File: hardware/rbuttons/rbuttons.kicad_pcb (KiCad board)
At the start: 2 copper layers, 62 x 105 mm, 8 parts, among them U1 SKRBAKE010, U2 SKRBAKE010, U3 SKRBAKE010, U4 SKRBAKE010, U5 SKRBAKE010

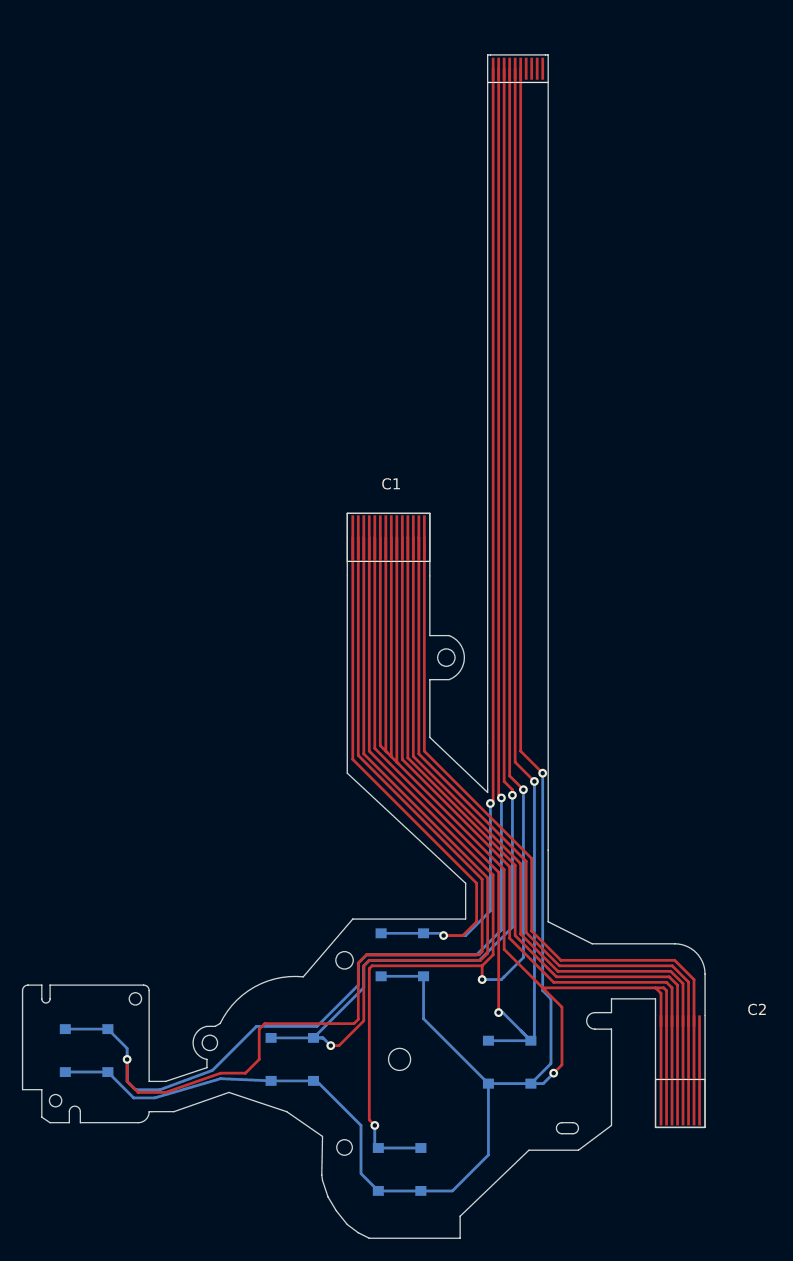
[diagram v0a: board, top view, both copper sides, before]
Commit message: Latest
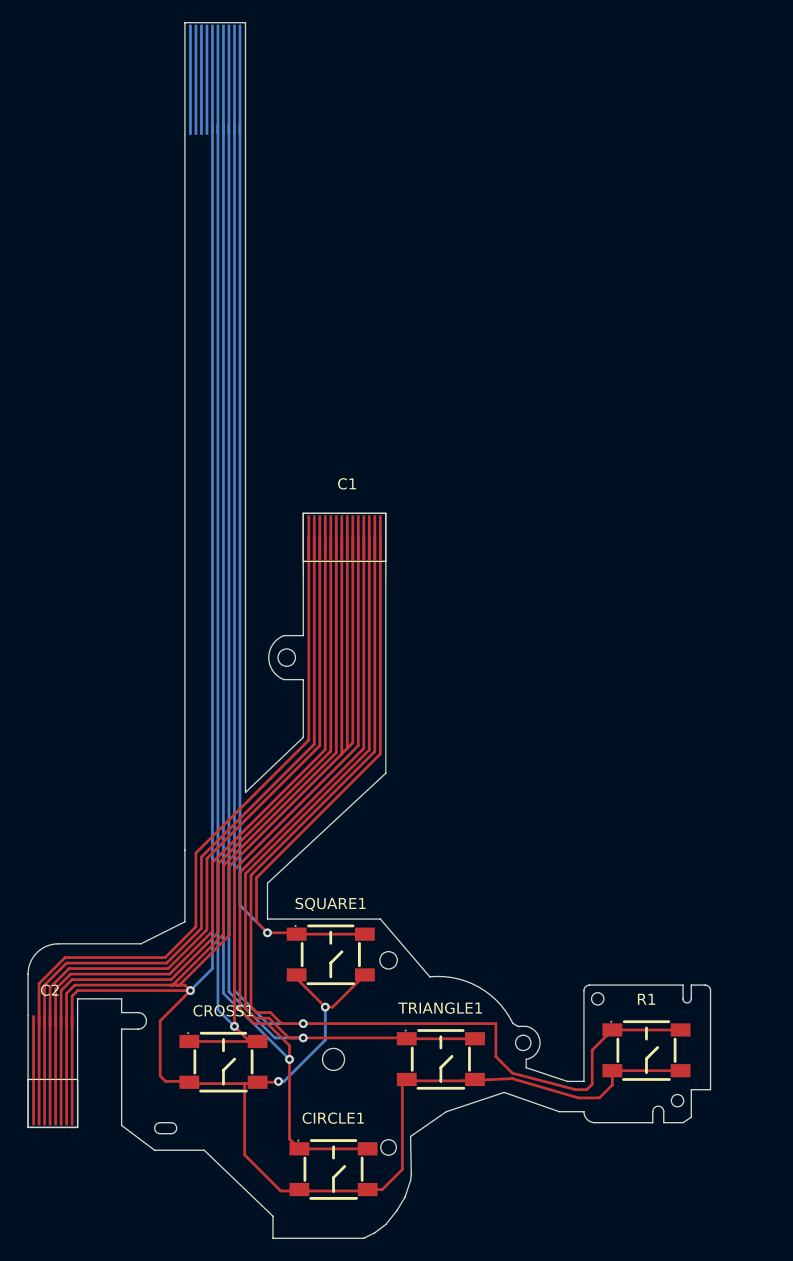
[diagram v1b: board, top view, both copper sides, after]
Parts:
- removed U1, U2, U3, U4, U5: SKRBAKE010, JLCPCB_footprint:KEY-SMD_4P-L4.0-W4.8-P3.90-LS4.8
- added CIRCLE1: K2-1187SQ-E4SW-06, JLCPCB_footprint:KEY-SMD_4P-L5.2-W5.2-P3.70-LS6.4, F.Cu at (97.5, 124.5)
- added CROSS1: K2-1187SQ-E4SW-06, JLCPCB_footprint:KEY-SMD_4P-L5.2-W5.2-P3.70-LS6.4, F.Cu at (87.5, 114.8)
- added R1: K2-1187SQ-E4SW-06, JLCPCB_footprint:KEY-SMD_4P-L5.2-W5.2-P3.70-LS6.4, F.Cu at (125.9, 113.7)
- added SQUARE1: K2-1187SQ-E4SW-06, JLCPCB_footprint:KEY-SMD_4P-L5.2-W5.2-P3.70-LS6.4, F.Cu at (97.2, 105.0)
- added TRIANGLE1: K2-1187SQ-E4SW-06, JLCPCB_footprint:KEY-SMD_4P-L5.2-W5.2-P3.70-LS6.4, F.Cu at (107.2, 114.5)
- C3: footprint consolizer:flex_short_10 -> consolizer:flex_long_10; moved to B.Cu
- moved C2 57.0 mm to (74.2, 107.4)
- moved C3 28.0 mm to (86.5, 24.5), turned to 180 degrees
- moved C1 4.00 mm to (98.6, 67.1)
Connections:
- C1 pad 1: /Square -> /five
- C1 pad 10: /one -> /cross
- C1 pad 11: /tw -> /Circle
- C1 pad 12: /three -> /Triangle
- C1 pad 13: /four -> /R1
- C1 pad 14: /five -> /Square
- C1 pad 2: /R1 -> /four
- C1 pad 3: /Triangle -> /three
- C1 pad 4: /Circle -> /tw
- C1 pad 5: /cross -> /one
- C2 pad 1: unconnected-(C2-Pad1) -> /gnd
- C2 pad 2: /five -> /gnd
- C2 pad 3: /four -> /one
- C2 pad 4: /three -> /tw
- C2 pad 5: /tw -> /three
- C2 pad 6: /one -> /four
- C2 pad 7: /gnd -> /five
- C2 pad 8: /gnd -> unconnected-(C2-Pad8)
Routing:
- net /R1: track 215.2 -> 181.1 mm, vias 2 -> 1
- net /gnd: track 304.9 -> 336.6 mm, vias 2 -> 3
- net /Triangle: track 171.3 -> 156.9 mm, vias 2 -> 1
- net /Square: track 130.7 -> 124.4 mm, vias 2 -> 1
- net /cross: track 146.2 -> 140.6 mm, vias 2 -> 1
- net /Circle: track 161.9 -> 156.9 mm, vias 3 -> 1
- net /one: track 60.6 -> 59.8 mm
- net /tw: track 60.6 -> 59.8 mm
- net /five: track 60.6 -> 59.9 mm
- net /three: track 60.6 -> 59.8 mm
- net /four: track 60.6 -> 59.9 mm
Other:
- board size 62 x 105 mm -> 62 x 100.2 mm
